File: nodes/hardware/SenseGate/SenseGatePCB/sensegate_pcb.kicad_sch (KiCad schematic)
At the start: 33 parts, among them J10 Conn_01x02_Pin, J3 Conn_01x02_Socket, J4 Conn_01x24_Pin, J5 Conn_01x04_Socket, J6 Conn_01x04_Socket, J7 Conn_01x04_Socket, J8 Conn_01x04_Socket, J9 Conn_01x04_Socket, Q4 SS8050, SW1 SW_Reed, SW2 SW_Reed, SW3 SW_Reed, SW5 SW_DPDT_x2, U1 DD05CVSA, U2 mt3608_dcdc_converter

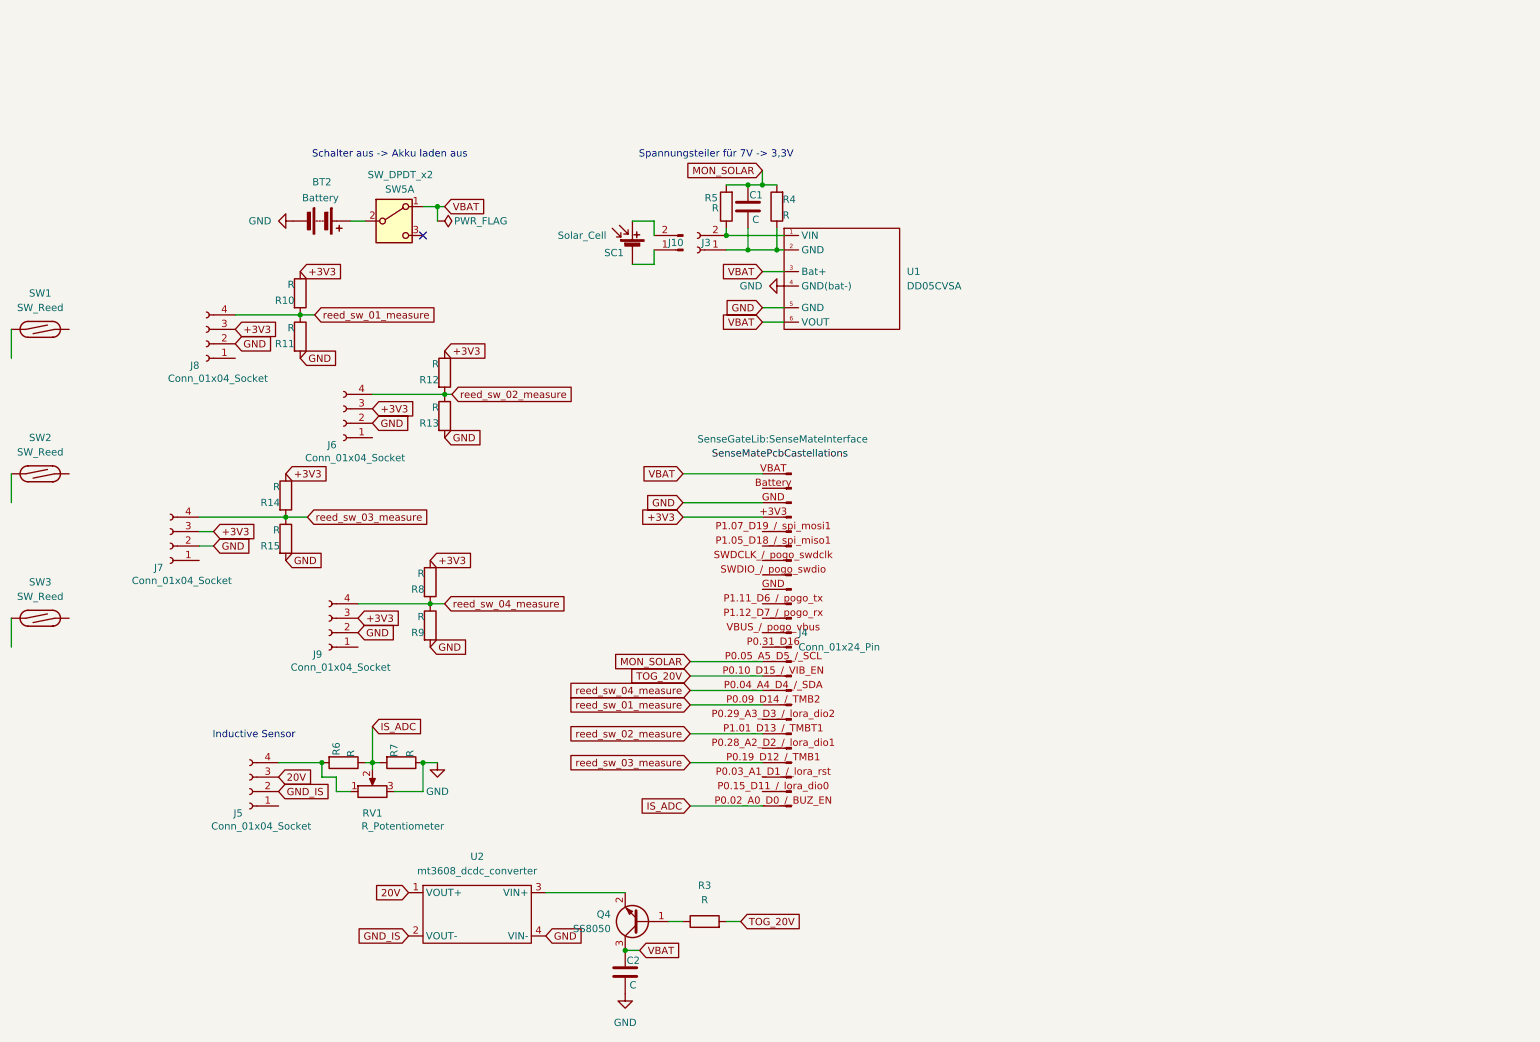
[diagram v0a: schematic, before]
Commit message: sensegate pcb v1 done?!
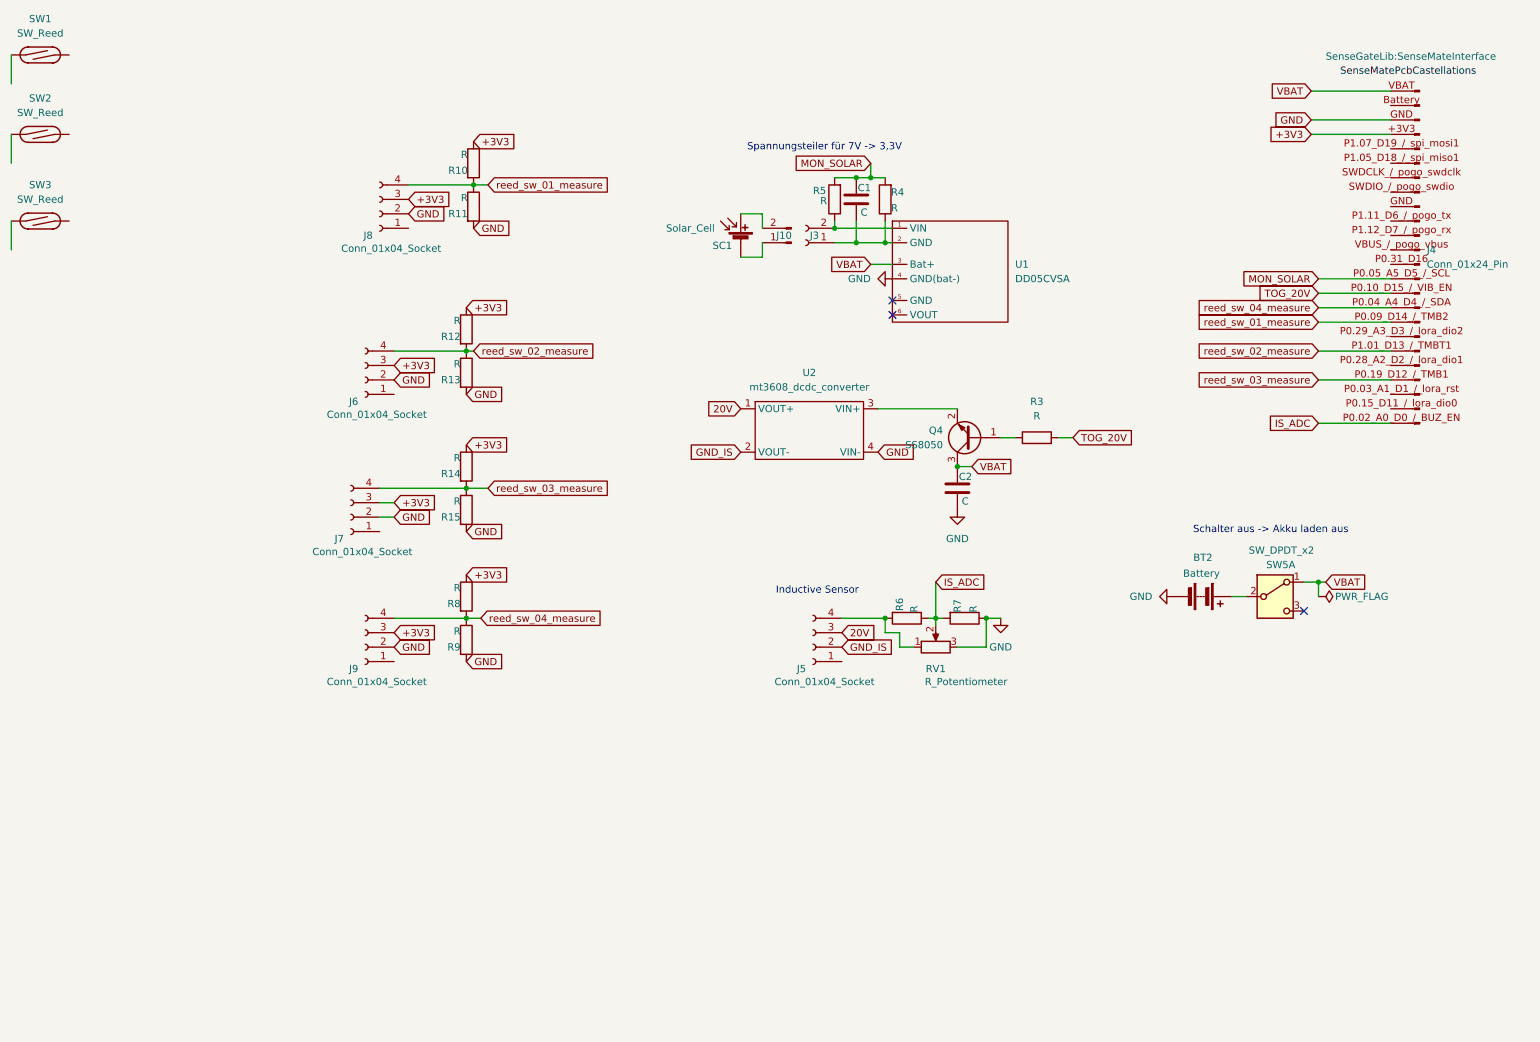
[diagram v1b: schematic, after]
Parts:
- C1, C2: footprint (none) -> Capacitor_THT:CP_Axial_L10.0mm_D6.0mm_P15.00mm_Horizontal
- RV1: footprint (none) -> Potentiometer_THT:Potentiometer_Bourns_3266W_Vertical
- SW5: footprint SenseMateLibrary:OS102011MA1QN1 -> SenseGateLib:OS102011MA1QN1
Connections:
- net GND: no longer U1.5 (GND)
- net VBAT: no longer U1.6 (VOUT)
- no-connect marks 1 -> 3
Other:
- moved on the sheet: BT2, C1, C2, J10, J3, J4, J5, J6, J7, J8, J9, Q4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
